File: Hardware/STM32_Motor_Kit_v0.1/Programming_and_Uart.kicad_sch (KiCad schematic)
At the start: 6 parts, among them J2 Conn_02x04_Odd_Even

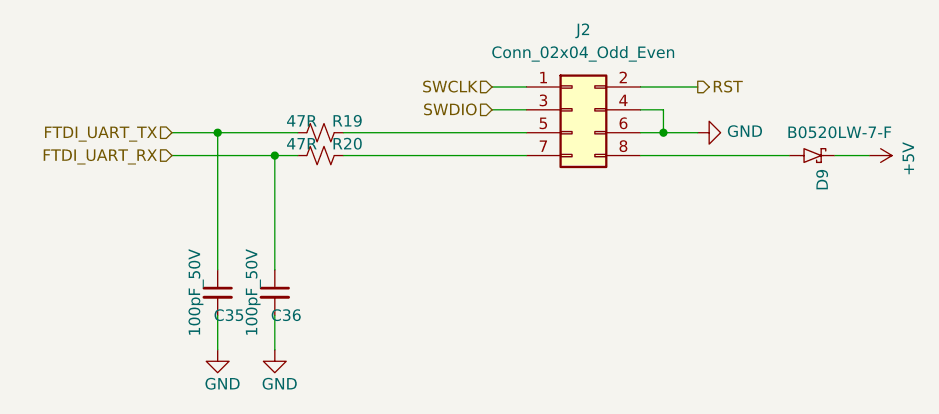
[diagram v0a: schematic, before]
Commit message: 12.01.2025
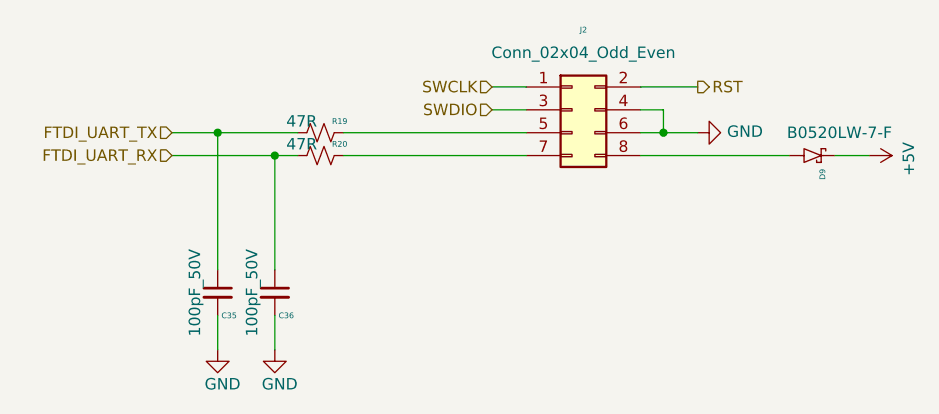
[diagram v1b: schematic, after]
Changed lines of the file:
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@@
 			(effects
 				(font
-					(size 1.27 1.27)
+					(face "Arial")
+					(size 0.635 0.635)
 				)
 				(justify left)
@@
 			(effects
 				(font
-					(size 1.27 1.27)
+					(face "Arial")
+					(size 0.635 0.635)
 				)
 			)
@@
 			(effects
 				(font
-					(size 1.27 1.27)
+					(face "Arial")
+					(size 0.635 0.635)
 				)
 			)
@@
 			(effects
 				(font
-					(size 1.27 1.27)
+					(face "Arial")
+					(size 0.635 0.635)
 				)
 				(hide yes)
@@
 			(effects
 				(font
-					(size 1.27 1.27)
+					(face "Arial")
+					(size 0.635 0.635)
 				)
 			)
@@
 			(effects
 				(font
-					(size 1.27 1.27)
+					(face "Arial")
+					(size 0.635 0.635)
 				)
 				(hide yes)
@@
 			(effects
 				(font
-					(size 1.27 1.27)
+					(face "Arial")
+					(size 0.635 0.635)
 				)
 				(hide yes)
@@
 			(effects
 				(font
-					(size 1.27 1.27)
+					(face "Arial")
+					(size 0.635 0.635)
 				)
 				(justify left)
@@
 			(effects
 				(font
-					(size 1.27 1.27)
+					(face "Arial")
+					(size 0.635 0.635)
 				)
 				(justify left)
@@
 			(effects
 				(font
-					(size 1.27 1.27)
-				)
-				(hide yes)
+					(face "Arial")
+					(size 0.635 0.635)
+				)
+				(hide yes)
